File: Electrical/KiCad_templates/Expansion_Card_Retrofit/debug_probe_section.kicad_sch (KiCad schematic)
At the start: 15 parts, among them U3 W25Q16JVUXIQ, U4 RP2040

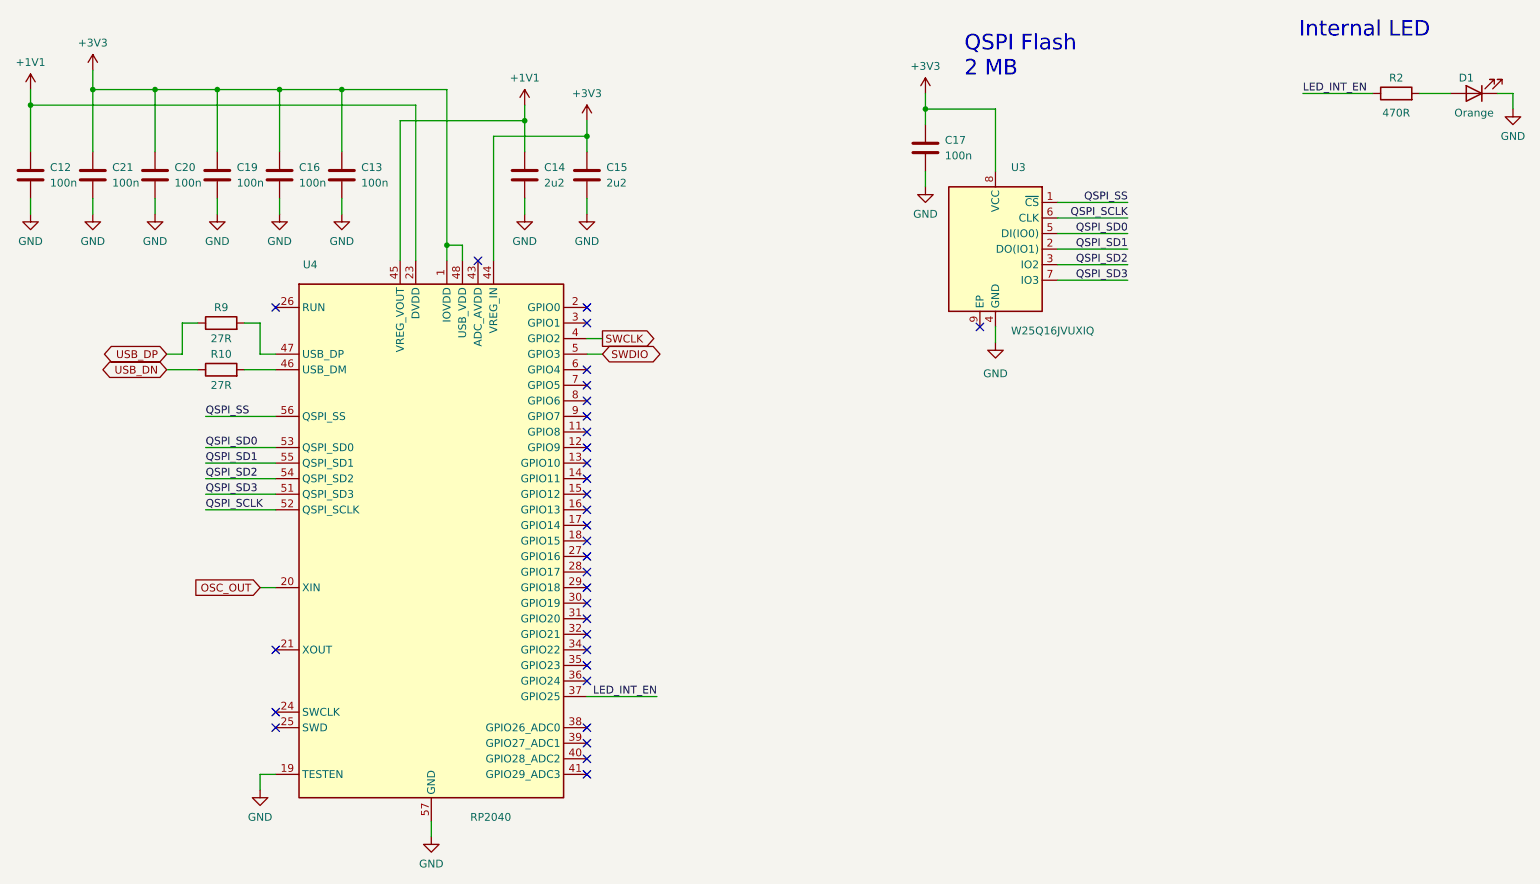
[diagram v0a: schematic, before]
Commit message: Current state before flash footprint update
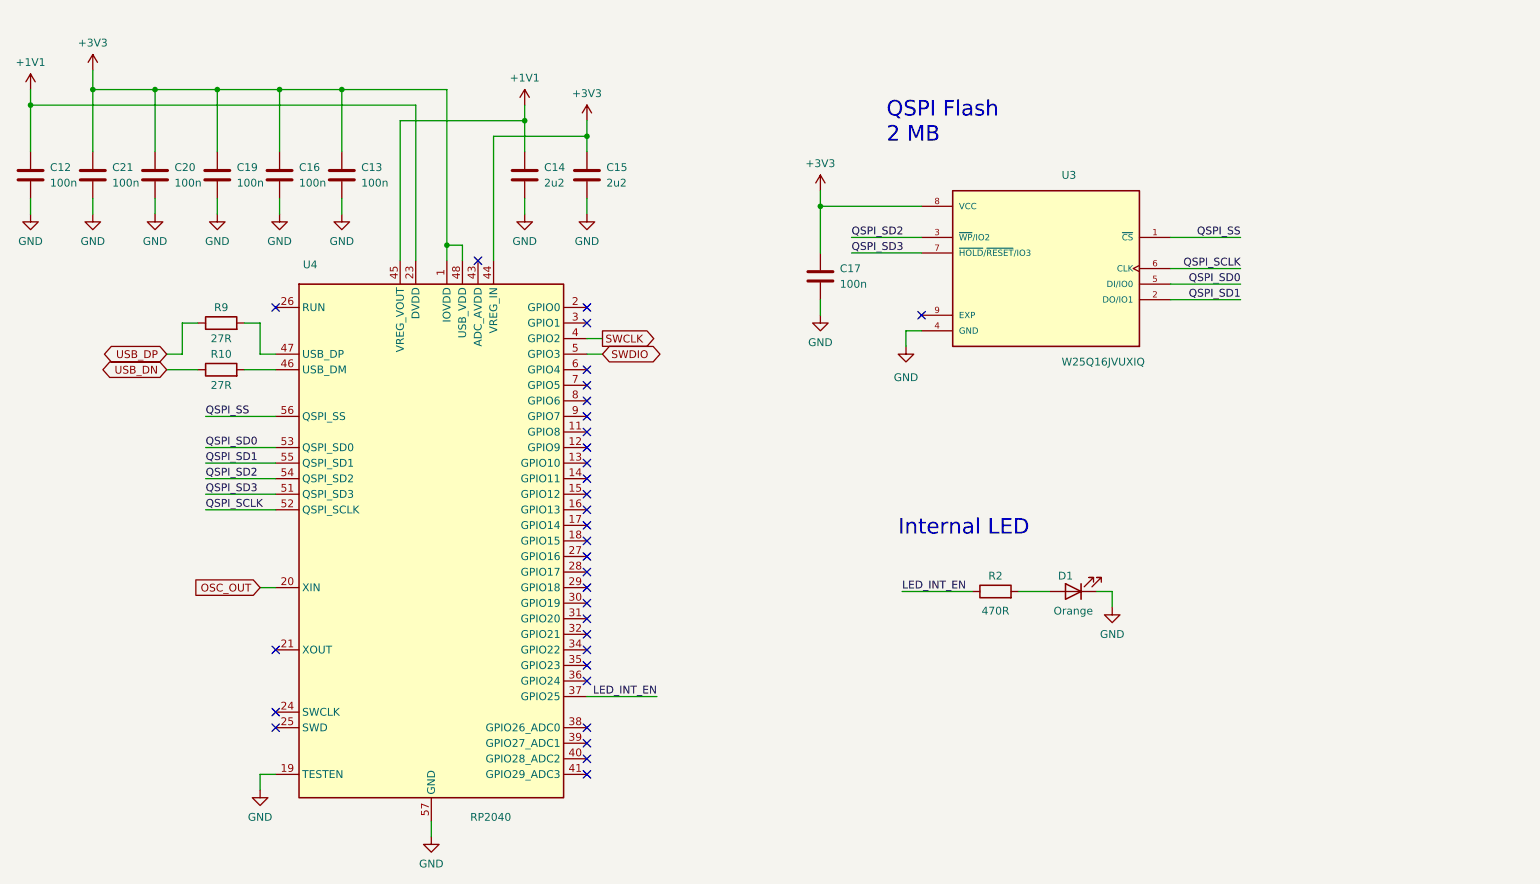
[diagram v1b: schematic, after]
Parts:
- U3: footprint Package_SON:WSON-8-1EP_6x5mm_P1.27mm_EP3.4x4.3mm -> SnapEDA:IC_W25Q16JVUXIQ_TR; symbol Memory_Flash:W25Q32JVZP -> SnapEDA:W25Q16JVUXIQ_TR; Availability (none) -> In Stock; Check_prices (none) -> https://www.snapeda.com/parts/W25Q16JVUXIQ%20TR/Winbond/vie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; MANUFACTURER (none) -> Winbond; MAXIMUM_PACKAGE_HEIGHT (none) -> 0.60mm; MF (none) -> Winbond; MP (none) -> W25Q16JVUXIQ TR; PARTREV (none) -> H; Package (none) -> UFDFN-8 Winbond; Price (none) -> None; Purchase-URL (none) -> https://www.snapeda.com/api/url_track_click_mouser/?unipart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; SNAPEDA_PN (none) -> W25Q16JVUXIQ TR; STANDARD (none) -> Manufacturer Recommendations; SnapEDA_Link (none) -> https://www.snapeda.com/parts/W25Q16JVUXIQ%20TR/Winbond/vie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
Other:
- moved on the sheet: C17, D1, R2
